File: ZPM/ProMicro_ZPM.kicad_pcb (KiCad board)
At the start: 2 copper layers, 17.8 x 30.5 mm, 17 parts, among them J1 Screw_Terminal_01x05, J3 JST, Q1 BC847, U1 LTC3588EDD-1PBF, U2 MCP73831-2-OT

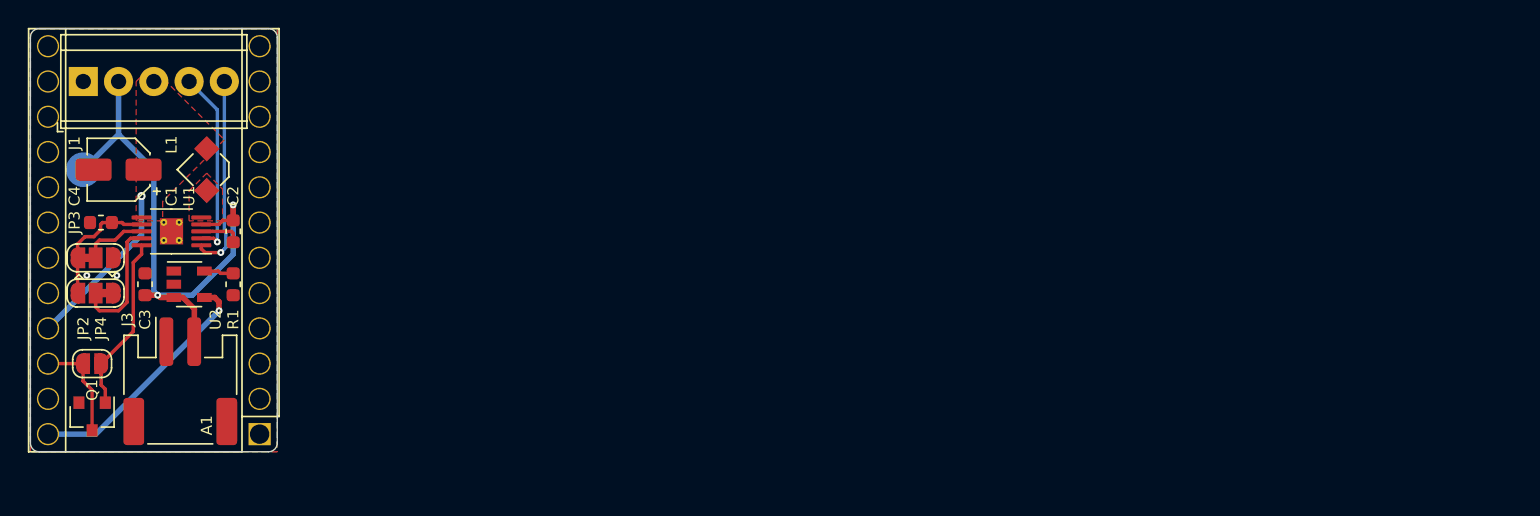
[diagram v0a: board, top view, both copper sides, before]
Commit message: ZPM
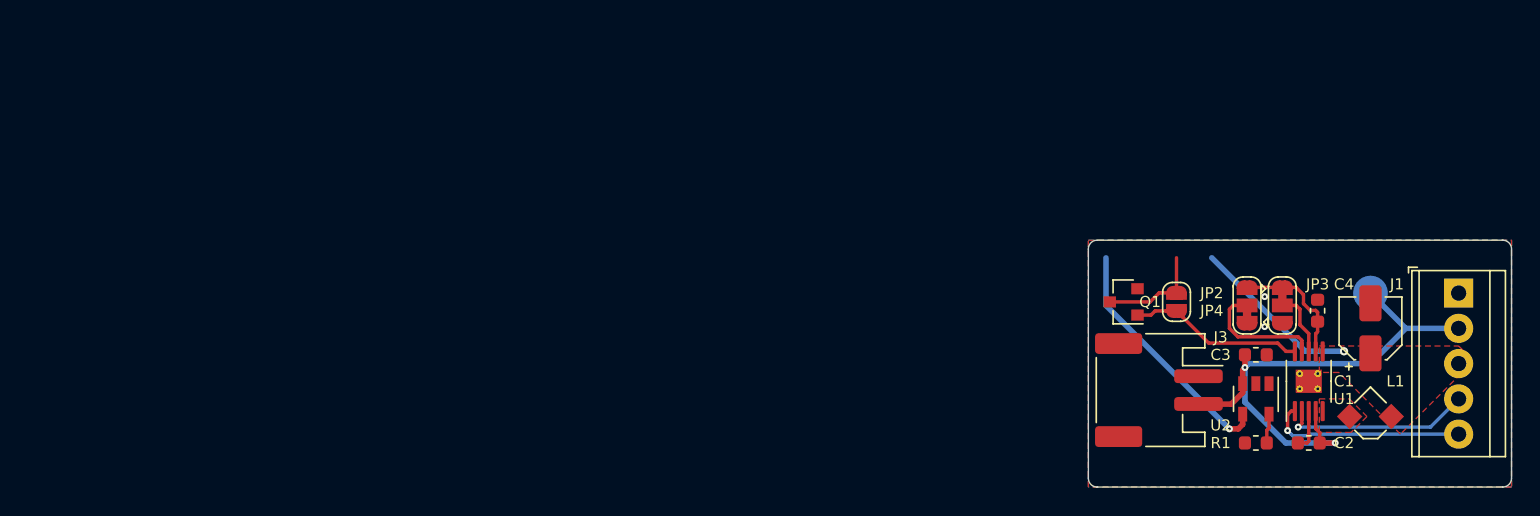
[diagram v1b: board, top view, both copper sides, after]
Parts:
- removed A1: Sparkfun_Pro_Micro_3V3, Module:Sparkfun_Pro_Micro
- moved J1 100.2 mm to (152.4, 94.0), turned to 270 degrees
- moved TP1 93.1 mm to (146.1, 94.0), turned to 270 degrees
- moved C1 90.9 mm to (146.1, 96.5), turned to 90 degrees
- moved C4 87.9 mm to (142.2, 95.2), turned to 90 degrees
- moved L1 85.7 mm to (146.1, 102.9), turned to 225 degrees
- moved JP3 85.5 mm to (139.7, 94.9), turned to 270 degrees
- moved JP2 82.9 mm to (137.2, 94.9), turned to 90 degrees
- moved U1 82.6 mm to (141.6, 100.3), turned to 90 degrees
- moved C3 80.2 mm to (137.8, 98.4), turned to 0 degrees
- moved C2 79.0 mm to (141.6, 104.8), turned to 0 degrees
- moved LOGO1 78.7 mm to (139.1, 101.6), turned to 180 degrees
- moved JP4 78.2 mm to (132.1, 94.6), turned to 270 degrees
- moved U2 77.3 mm to (137.8, 101.6), turned to 270 degrees
- moved Q1 74.8 mm to (128.3, 94.6), turned to 180 degrees
- moved R1 74.5 mm to (137.8, 104.8), turned to 180 degrees
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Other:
- board size 17.8 x 30.5 mm -> 30.5 x 17.8 mm
